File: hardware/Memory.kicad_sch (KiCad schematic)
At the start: 13 parts, among them J15 Micro_SD_Card_Det_Hirose_DM3AT, U20 AT45DB641E-SHN-T

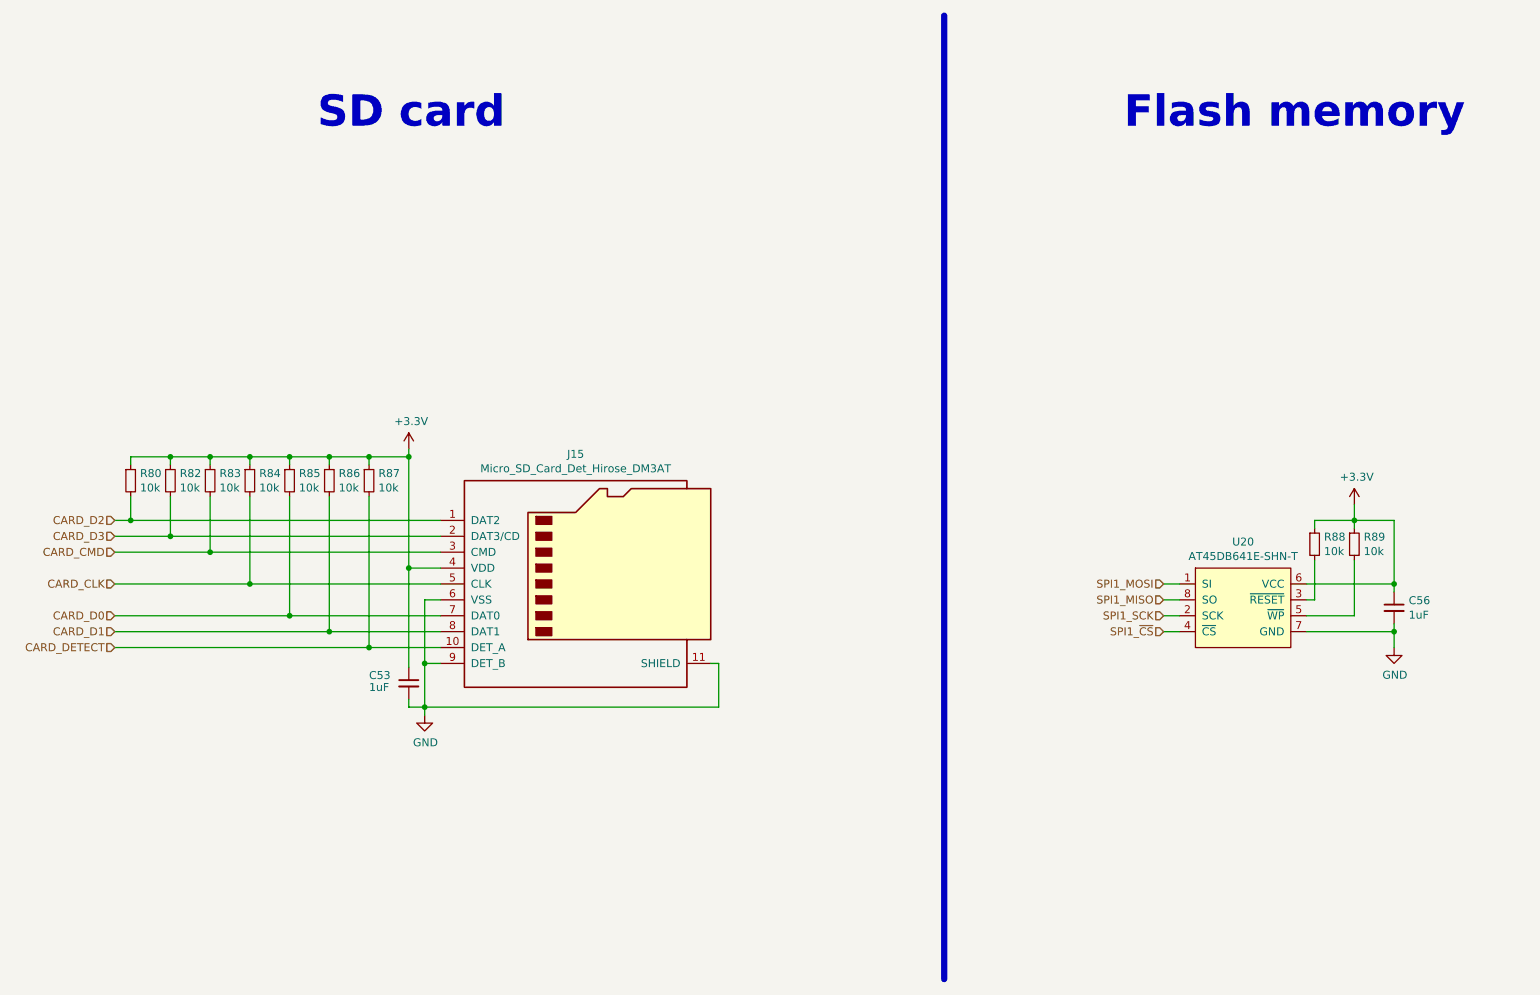
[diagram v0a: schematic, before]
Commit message: schematic override, just cuz
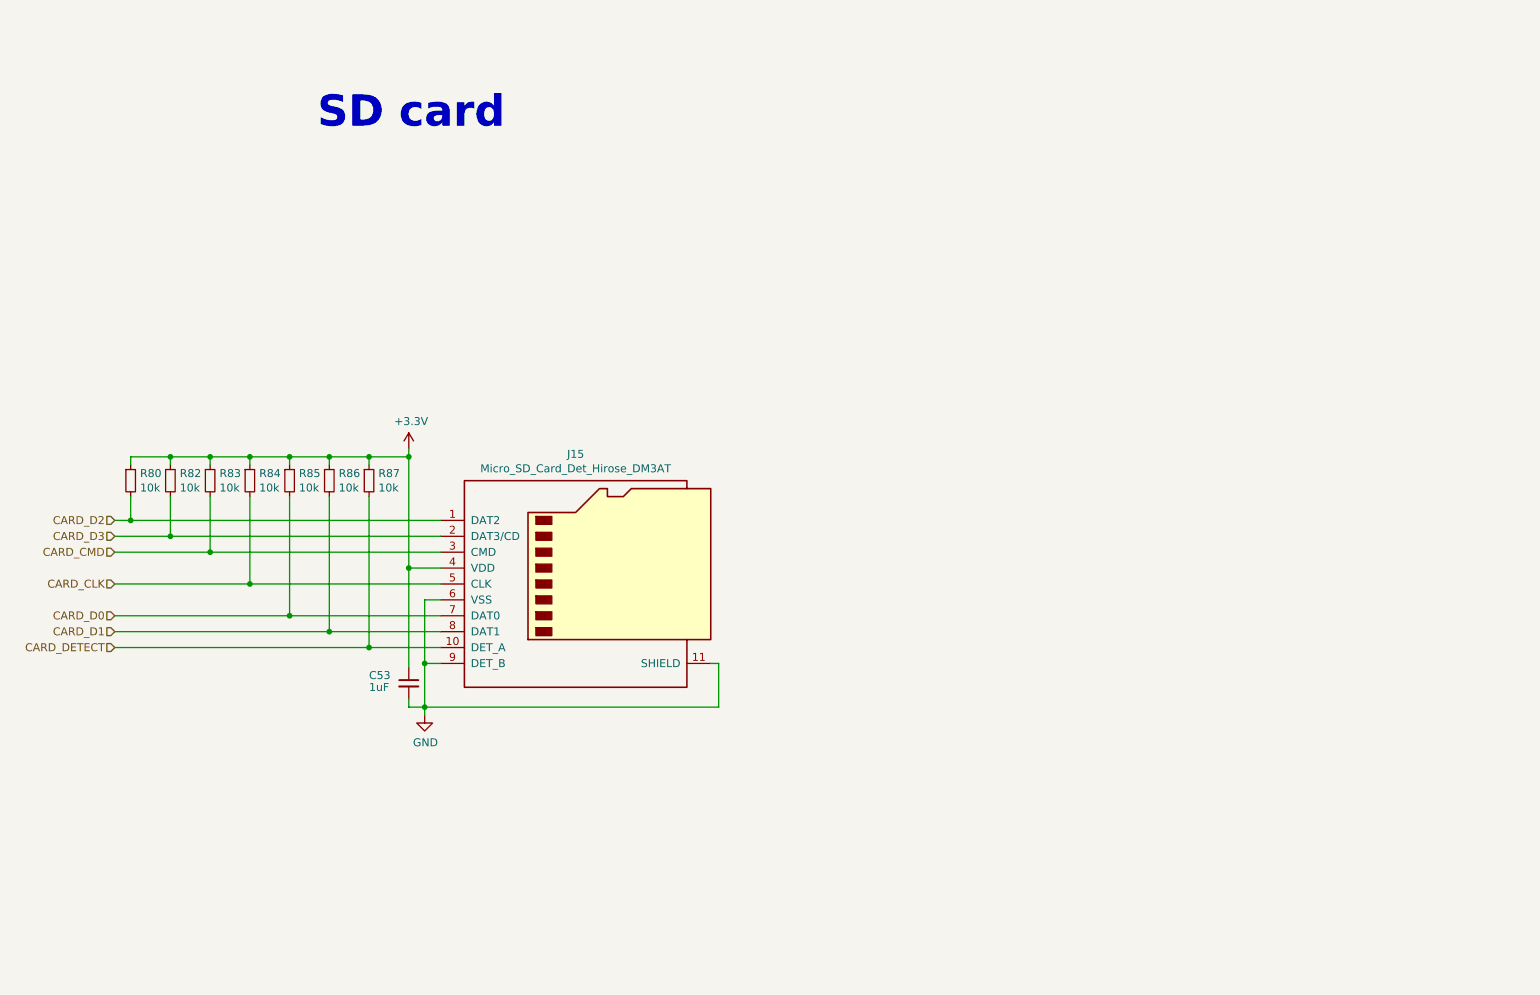
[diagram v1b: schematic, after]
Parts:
- removed C56: 1uF, Capacitor_SMD:C_0603_1608Metric, symbol Device:C_Small
- removed R88, R89: 10k, Resistor_SMD:R_0603_1608Metric, symbol Device:R_Small
- removed U20: AT45DB641E-SHN-T, Package_SO:SOIC-8_5.23x5.23mm_P1.27mm, symbol PUTM_EV_BMS_library:AT45DB641E-SHN-T
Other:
- note removed: "Flash memory"

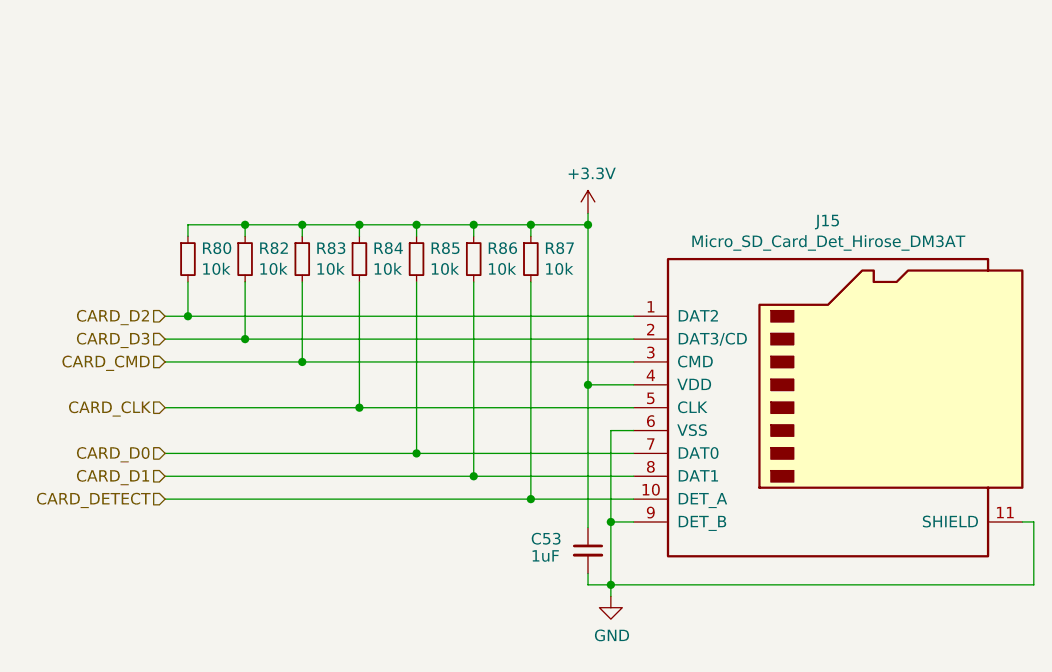
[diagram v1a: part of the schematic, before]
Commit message: remake in progress
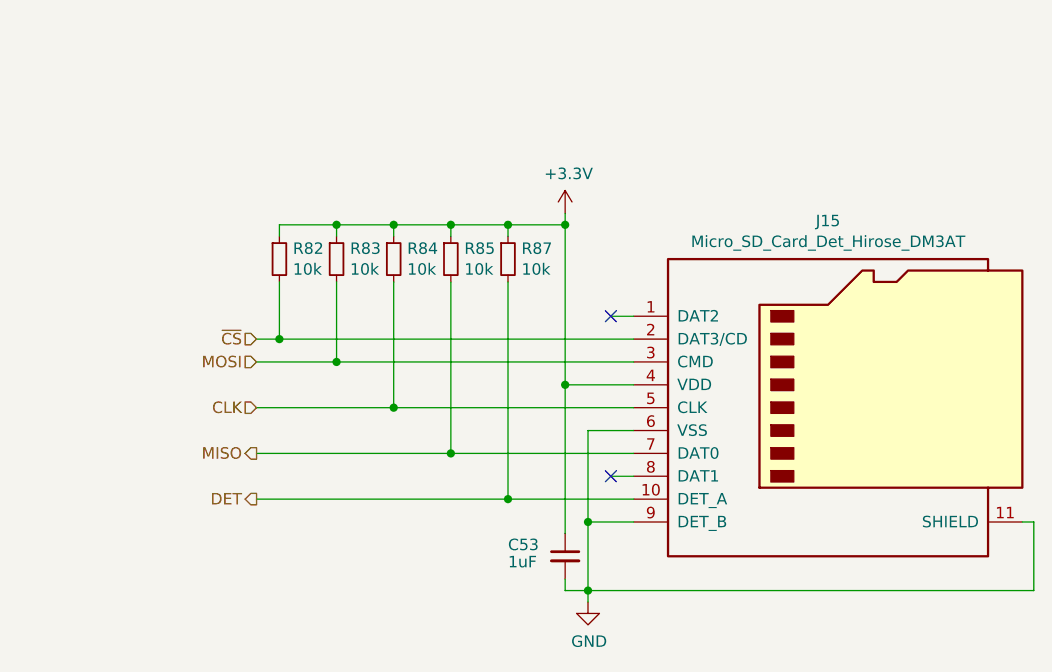
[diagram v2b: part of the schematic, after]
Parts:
- removed R80, R86: 10k, Resistor_SMD:R_0603_1608Metric, symbol Device:R_Small
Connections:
- net CARD_CLK renamed CLK
- net CARD_CMD renamed MOSI
- net CARD_D0 renamed MISO
- net CARD_D1: no longer names the net of J15.8 (DAT1)
- net CARD_D2: no longer names the net of J15.1 (DAT2)
- net CARD_D3 renamed ~{CS}
- net CARD_DETECT renamed DET
- no-connect marks 0 -> 2
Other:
- moved on the sheet: C53, R82, R83, R84, R85, R87
